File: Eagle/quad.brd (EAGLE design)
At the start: 100 x 60 mm, 15 parts

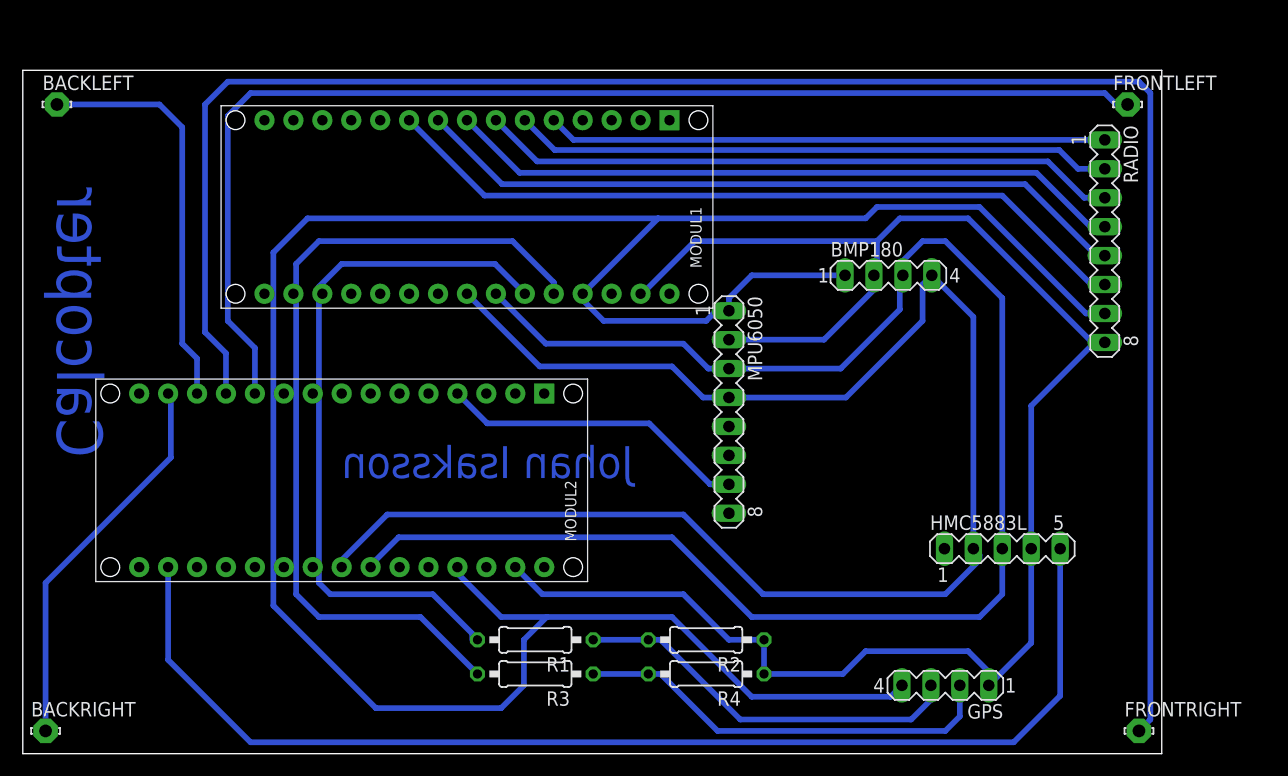
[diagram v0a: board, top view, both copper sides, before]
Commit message: Final board design and added ground fill.
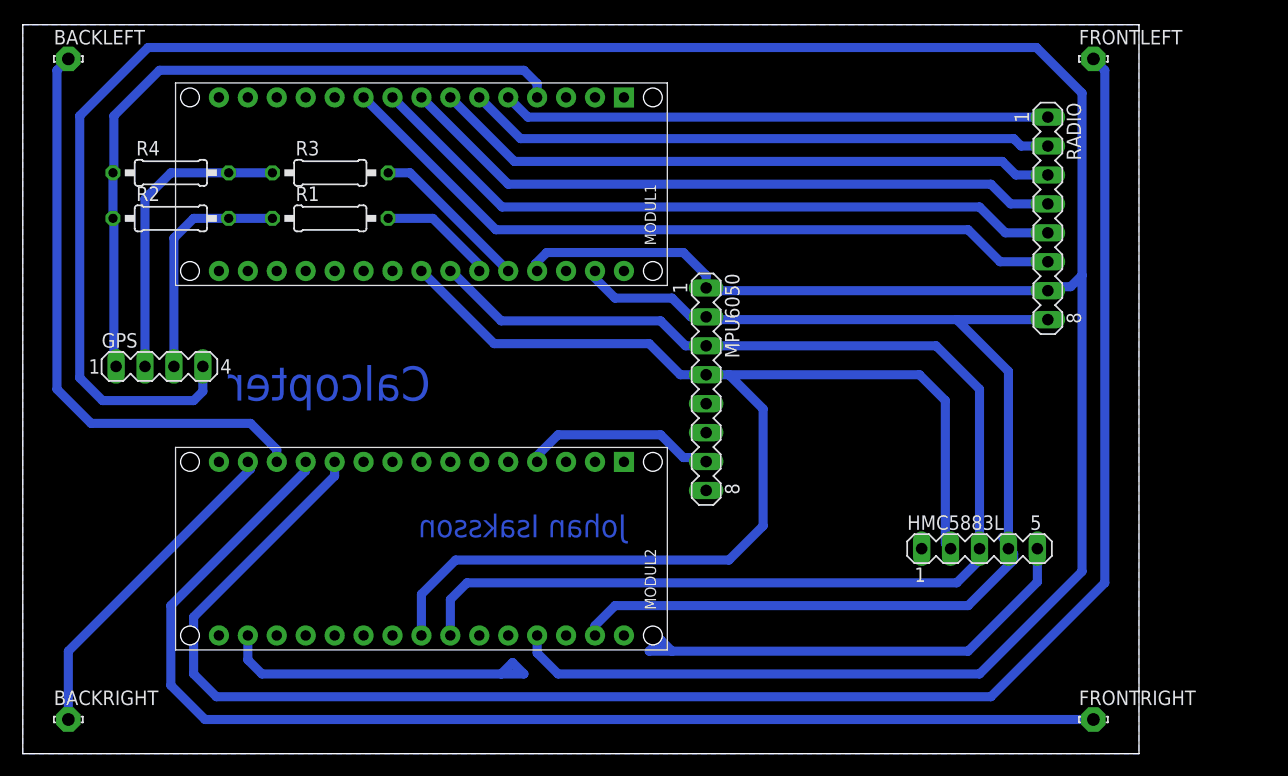
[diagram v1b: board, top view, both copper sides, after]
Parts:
- removed BMP180: (no value), con-lstb:MA04-1
- moved GPS 74.5 mm to (12.0, 34.0), turned to 0 degrees
- moved R4 64.4 mm to (13.0, 51.0), turned to 0 degrees
- moved R2 59.8 mm to (13.0, 47.0), turned to 0 degrees
- moved R3 47.5 mm to (27.0, 51.0), turned to 0 degrees
- moved R1 41.1 mm to (27.0, 47.0), turned to 0 degrees
- moved MODUL2 9.22 mm to (35.0, 18.0)
- moved RADIO 5.39 mm to (90.0, 47.0)
- moved FRONTLEFT 5.00 mm to (94.0, 61.0)
- moved MODUL1 4.47 mm to (35.0, 50.0)
- moved BACKLEFT 4.12 mm to (4.00, 61.0)
- moved FRONTRIGHT 4.12 mm to (94.0, 3.00)
- moved MPU6050 2.83 mm to (60.0, 32.0)
- moved BACKRIGHT 2.24 mm to (4.00, 3.00)
- moved HMC5883L 2.00 mm to (84.0, 18.0)
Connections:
- removed net COM: MODUL1.J1.4
- removed net N$2: BMP180.1, GPS.4, MODUL1.J2.4, MODUL2.J2.4, MPU6050.1, RADIO.7
- removed net N$9: BMP180.2, GPS.1, HMC5883L.4, MODUL1.J2.2, MODUL2.J1.4, MODUL2.J2.2, MPU6050.2, MPU6050.7, R2.1, R4.1, RADIO.8
- new net GND: GPS.1, HMC5883L.4, MODUL1.J1.4, MODUL1.J2.2, MODUL2.J1.4, MODUL2.J2.2, MPU6050.2, MPU6050.7, R2.1, R4.1, RADIO.8
- new net VDD: GPS.4, MODUL1.J2.4, MODUL2.J2.4, MPU6050.1, RADIO.7
- net N$16: no longer BMP180.3
- net N$17: no longer BMP180.4
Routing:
- net VDD: track 0.00 -> 276.9 mm
- net N$2: track 223.7 -> 0.00 mm
- net GND: track 0.00 -> 185.8 mm
- net N$9: track 179.4 -> 0.00 mm
- net N$6: track 166.8 -> 106.8 mm
- net N$18: track 73.8 -> 14.1 mm
- net N$10: track 61.8 -> 10.2 mm
- net N$1: track 105.6 -> 155.1 mm
- net N$14: track 104.1 -> 72.1 mm
- net N$16: track 143.7 -> 116.8 mm
- net N$17: track 141.1 -> 114.5 mm
- net N$3: track 35.7 -> 52.0 mm
- net N$20: track 34.5 -> 20.6 mm
- net N$21: track 37.5 -> 26.9 mm
- net N$4: track 34.4 -> 29.3 mm
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- added copper zone on layer 16, net GND
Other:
- board size 100 x 60 mm -> 98 x 64 mm
